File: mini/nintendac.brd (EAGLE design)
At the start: 26 x 42 mm, 30 parts, among them IC1 STM32F10XCXT6, IC3 24C64ST, X1 USB-MICROB

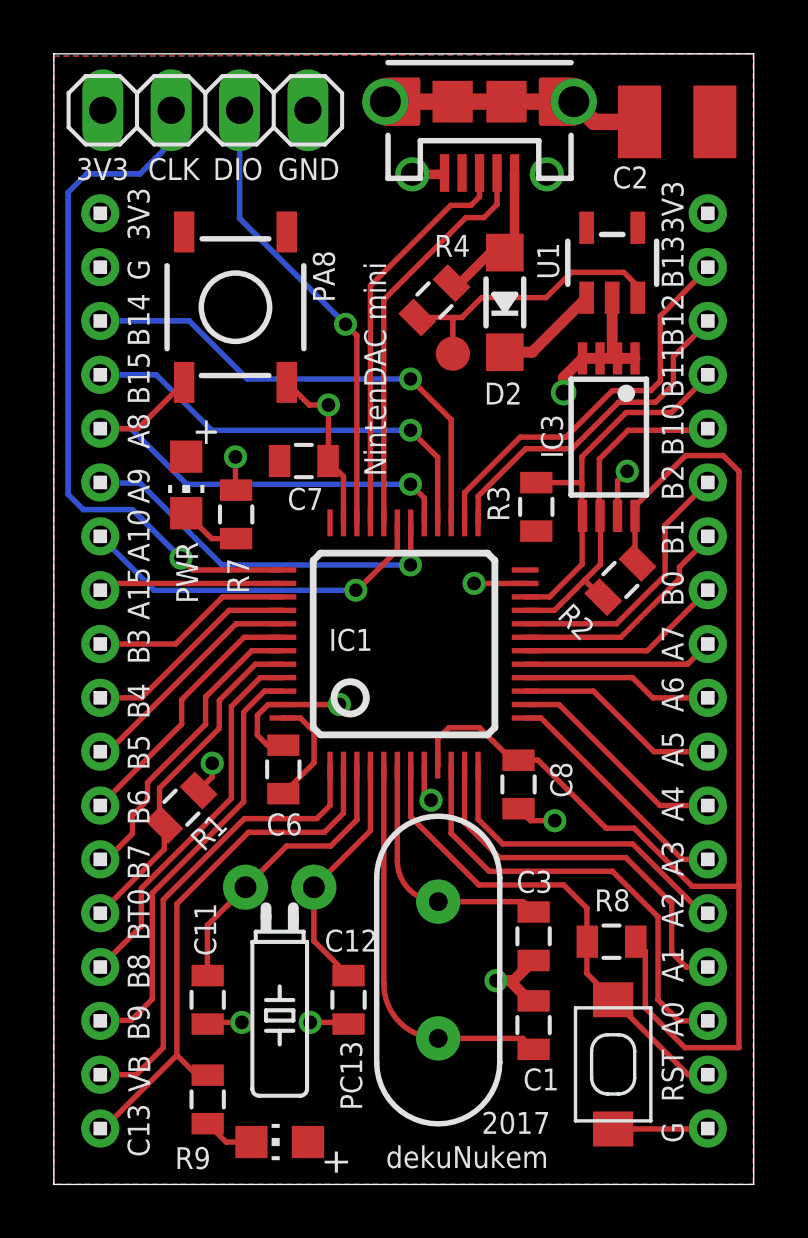
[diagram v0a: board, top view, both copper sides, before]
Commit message: board cleanup
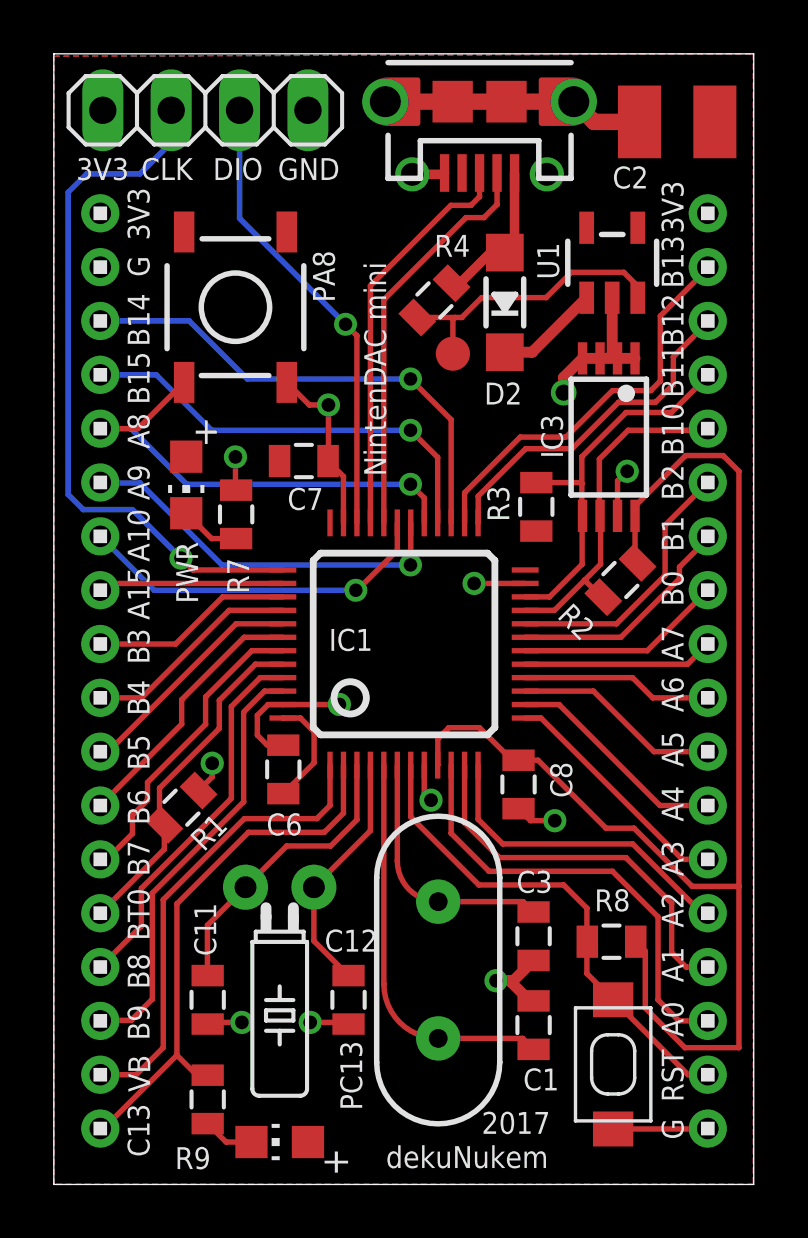
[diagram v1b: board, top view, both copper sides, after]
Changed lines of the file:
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@@
 <text x="2.7686" y="4.81" size="0.8128" layer="25" rot="R270">VB</text>
 <text x="0.8288" y="37.3126" size="0.8128" layer="25">3V3</text>
-<text x="3.4958" y="37.3126" size="0.8128" layer="25">CLK</text>
+<text x="3.2418" y="37.3126" size="0.8128" layer="25">CLK</text>
 <text x="5.9088" y="37.3126" size="0.8128" layer="25">DIO</text>
 <text x="8.3218" y="37.3126" size="0.8128" layer="25">GND</text>
@@
 <text x="2.7432" y="8.5852" size="0.8128" layer="25" distance="10" rot="R270">B8</text>
 <text x="2.7432" y="10.9982" size="0.8128" layer="25" distance="10" rot="R270">BT0</text>
-<text x="2.7432" y="12.6492" size="0.8128" layer="25" distance="10" rot="R270">B7</text>
+<text x="2.7432" y="12.7762" size="0.8128" layer="25" distance="10" rot="R270">B7</text>
 <text x="2.7432" y="14.6812" size="0.8128" layer="25" distance="10" rot="R270">B6</text>
 <text x="2.7432" y="16.7132" size="0.8128" layer="25" distance="10" rot="R270">B5</text>
-<text x="2.7432" y="18.6182" size="0.8128" layer="25" distance="10" rot="R270">B4</text>
+<text x="2.7432" y="18.7452" size="0.8128" layer="25" distance="10" rot="R270">B4</text>
 <text x="2.7432" y="20.6502" size="0.8128" layer="25" distance="10" rot="R270">B3</text>
 <text x="2.7432" y="22.9362" size="0.8128" layer="25" distance="10" rot="R270">A15</text>
 <text x="2.7432" y="25.0952" size="0.8128" layer="25" distance="10" rot="R270">A10</text>
-<text x="2.7432" y="26.6192" size="0.8128" layer="25" distance="10" rot="R270">A9</text>
+<text x="2.7432" y="26.7462" size="0.8128" layer="25" distance="10" rot="R270">A9</text>
 <text x="2.7432" y="28.6512" size="0.8128" layer="25" distance="10" rot="R270">A8</text>
 <text x="2.7432" y="30.9372" size="0.8128" layer="25" distance="10" rot="R270">B15</text>
 <text x="2.7432" y="33.0962" size="0.8128" layer="25" distance="10" rot="R270">B14</text>
-<text x="2.7432" y="34.3662" size="0.8128" layer="25" distance="10" rot="R270">G</text>
+<text x="2.7432" y="34.4932" size="0.8128" layer="25" distance="10" rot="R270">G</text>
 <text x="2.7432" y="37.0332" size="0.8128" layer="25" distance="10" rot="R270">3V3</text>
-<text x="23.3934" y="1.54" size="0.8128" layer="25" rot="R90">G</text>
+<text x="23.3934" y="1.667" size="0.8128" layer="25" rot="R90">G</text>
 <text x="23.3934" y="3.064" size="0.8128" layer="25" rot="R90">RST</text>
 <text x="23.3934" y="5.477" size="0.8128" layer="25" rot="R90">A0</text>
@@
 <text x="23.3934" y="19.447" size="0.8128" layer="25" rot="R90">A7</text>
 <text x="23.3934" y="21.479" size="0.8128" layer="25" rot="R90">B0</text>
-<text x="23.3934" y="23.384" size="0.8128" layer="25" rot="R90">B1</text>
+<text x="23.3934" y="23.511" size="0.8128" layer="25" rot="R90">B1</text>
 <text x="23.3934" y="25.416" size="0.8128" layer="25" rot="R90">B2</text>
 <text x="23.3934" y="27.067" size="0.8128" layer="25" rot="R90">B10</text>
@@
 <wire x1="24.8666" y1="27.0764" x2="25.4508" y2="26.4922" width="0.2032" layer="1"/>
 <wire x1="17.9882" y1="15.759" x2="17.2626" y2="15.759" width="0.2032" layer="1"/>
+<wire x1="21.5904" y1="24.8372" x2="21.5904" y2="23.1831875" width="0.2032" layer="1"/>
 <wire x1="19.7924" y1="35.5393" x2="19.7772" y2="35.6108" width="0" layer="19" extent="1-1"/>
-<wire x1="21.5904" y1="24.8372" x2="21.5904" y2="23.1831875" width="0.2032" layer="1"/>
 </signal>
 <signal name="N$1">
